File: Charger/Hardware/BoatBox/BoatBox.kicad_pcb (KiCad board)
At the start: 2 copper layers, 119 parts, among them P101 TestPoint, P102 TestPoint, P103 TestPoint, P104 TestPoint, P105 TestPoint, P106 TestPoint, P107 TestPoint, P108 TestPoint, P109 TestPoint, P110 TestPoint, P111 TestPoint, P112 TestPoint, P113 TestPoint, P114 TestPoint, P115 TestPoint, P116 TestPoint, P117 TestPoint, P118 TestPoint, P119 TestPoint, P120 TestPoint, P201 TestPoint, P202 TestPoint, P301 TestPoint, P302 TestPoint, P401 TestPoint, P402 TestPoint, P501 TestPoint, P502 TestPoint, T101 IRFR5505PBF, T102 BSS138, T103 IRFR5505PBF, T201 BC847, T202 IPD50R380CE, T203 BSS138, T301 BC847, T302 IPD50R380CE, T303 BSS138, T401 BC847, T402 IPD50R380CE, T403 BSS138, T501 BC847, T502 IPD50R380CE, T503 BSS138, X101 HCCPHPE24BKA90F

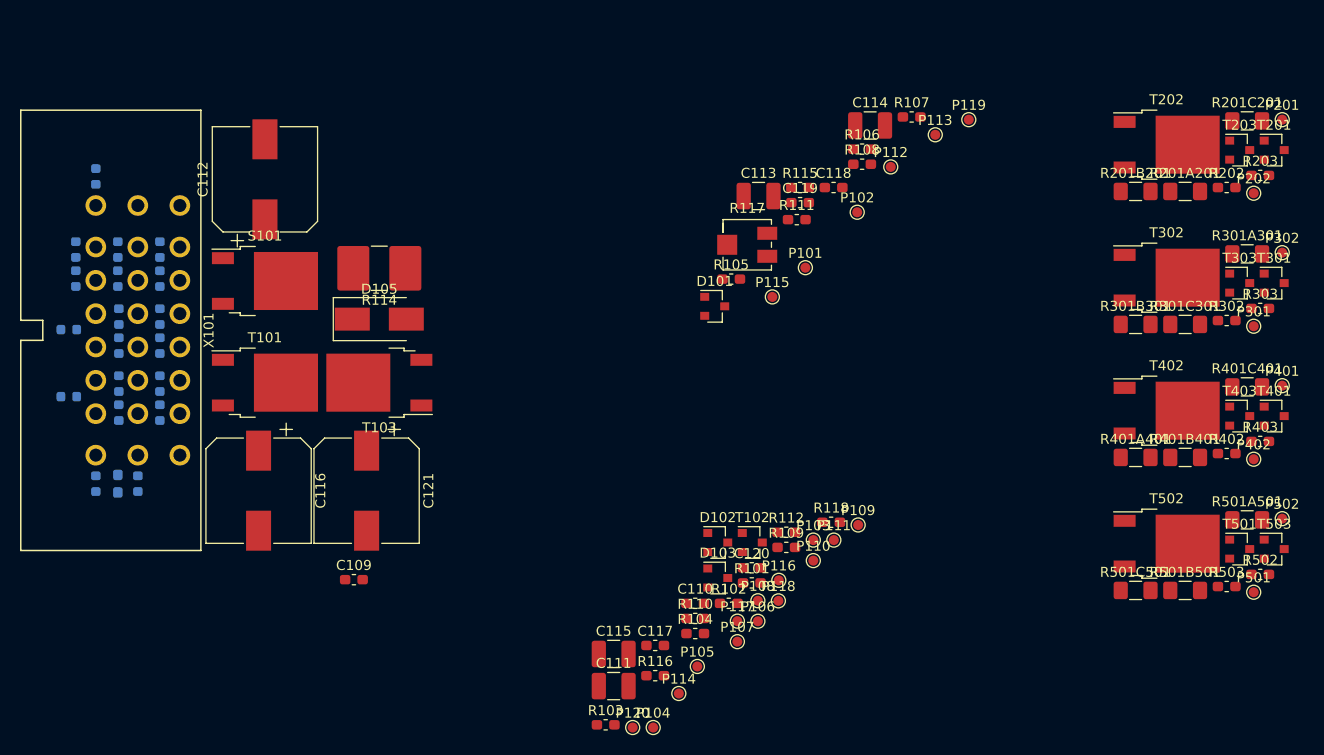
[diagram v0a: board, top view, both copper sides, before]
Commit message: WIP commit of new layout
squash after finish
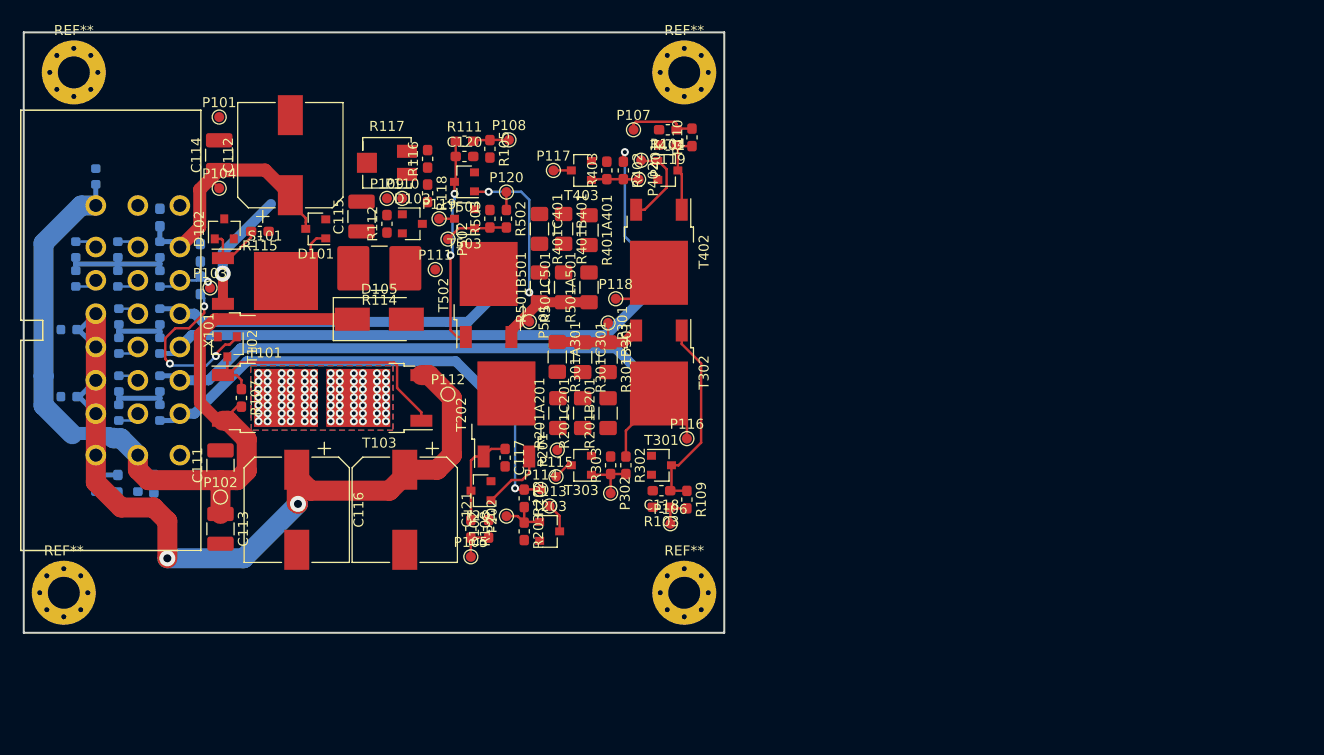
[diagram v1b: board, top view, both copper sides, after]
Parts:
- added REF**: MountingHole_3.2mm_M3_Pad_Via, MountingHole:MountingHole_3.2mm_M3_Pad_Via, F.Cu at (245.0, 211.0)
- added REF**: MountingHole_3.2mm_M3_Pad_Via, MountingHole:MountingHole_3.2mm_M3_Pad_Via, F.Cu at (245.0, 159.0)
- added REF**: MountingHole_3.2mm_M3_Pad_Via, MountingHole:MountingHole_3.2mm_M3_Pad_Via, F.Cu at (183.0, 211.0)
- added REF**: MountingHole_3.2mm_M3_Pad_Via, MountingHole:MountingHole_3.2mm_M3_Pad_Via, F.Cu at (184.0, 159.0)
- C109, C110, R101, R106: moved to B.Cu
- moved P502 87.9 mm to (221.4, 175.6), turned to 270 degrees
- moved T503 87.4 mm to (223.0, 173.6), turned to 180 degrees
- moved T201 86.3 mm to (224.7, 200.8), turned to 180 degrees
- moved T501 85.7 mm to (223.0, 169.9), turned to 180 degrees
- moved R502 83.3 mm to (227.2, 173.6), turned to 270 degrees
- moved R503 82.3 mm to (225.6, 173.6), turned to 90 degrees
- moved R203 81.7 mm to (229.0, 204.8), turned to 270 degrees
- moved P202 81.3 mm to (227.2, 203.3), turned to 90 degrees
- moved P201 79.6 mm to (232.3, 196.7), turned to 90 degrees
- moved T203 78.8 mm to (231.5, 204.8)
- moved P501 77.3 mm to (229.5, 183.9), turned to 270 degrees
- moved R202 76.8 mm to (229.0, 201.5), turned to 270 degrees
- moved R107 72.6 mm to (200.7, 191.5), turned to 270 degrees
- moved R201C201 72.5 mm to (234.8, 193.0), turned to 90 degrees
- moved R401C401 72.5 mm to (230.5, 174.6), turned to 270 degrees
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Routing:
- net UBD: track 0.00 -> 91.4 mm
- net UBR: track 0.00 -> 91.1 mm, vias 0 -> 2
- net /A_T_OUT3: track 0.00 -> 67.5 mm, vias 0 -> 1
- net /A_T_OUT2: track 0.00 -> 64.3 mm
- net /A_T_OUT1: track 0.00 -> 45.5 mm, vias 0 -> 1
- net /U_U_CHRG: track 0.00 -> 38.6 mm, vias 0 -> 1
- net /A_T_OUT4: track 0.00 -> 36.1 mm
- net Net-(R107-Pad1): track 0.00 -> 29.5 mm
- net Net-(P501-Pad1): track 0.00 -> 28.4 mm, vias 0 -> 2
- net GND: track 0.00 -> 25.9 mm
- net /LSS 4/ctrl: track 0.00 -> 20.9 mm, vias 0 -> 2
- net /LSS 2/ctrl: track 0.00 -> 20.2 mm
- net Net-(R106-Pad2): track 0.00 -> 17.8 mm, vias 0 -> 3
- net Net-(P301-Pad1): track 0.00 -> 10.3 mm
- net /LSS 1/ctrl: track 0.00 -> 9.85 mm
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- added copper zone on B.Cu, net Net-(T101-Pad2)
- added copper zone on F.Cu, net Net-(T101-Pad2)
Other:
- board outline added: 70 x 60 mm
